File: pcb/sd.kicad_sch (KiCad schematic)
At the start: 1 part

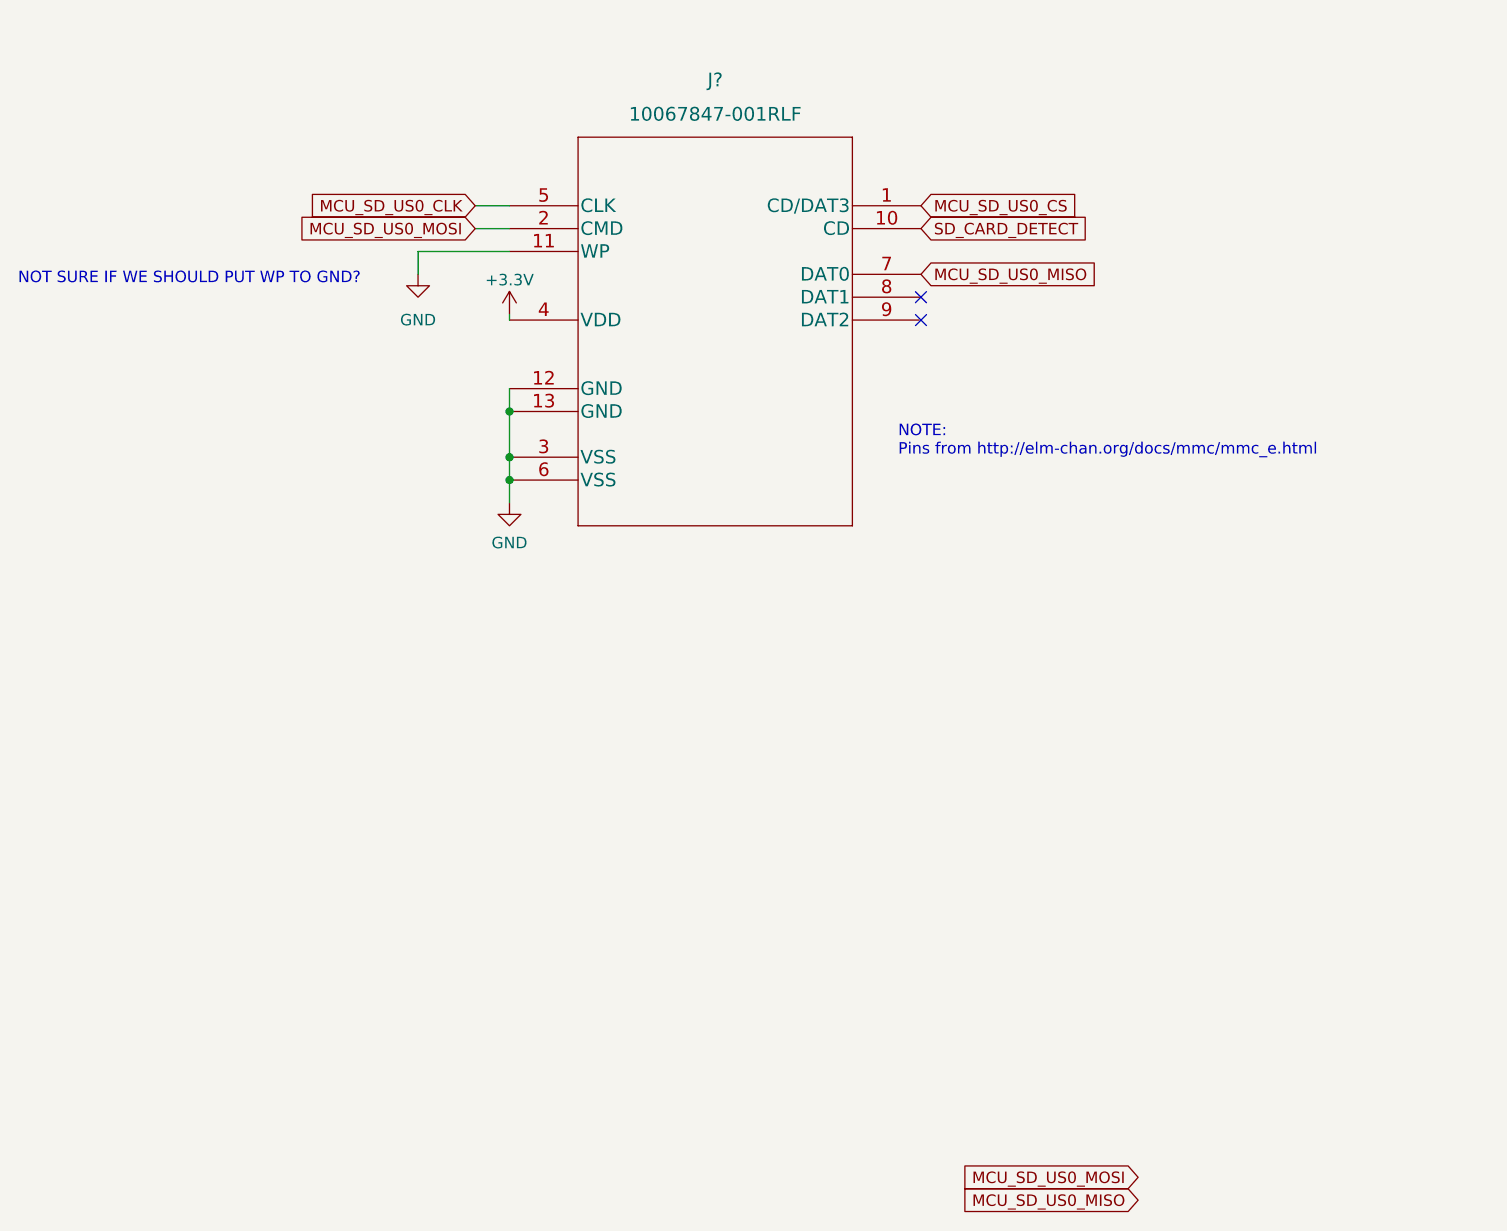
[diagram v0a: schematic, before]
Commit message: everything except crystal
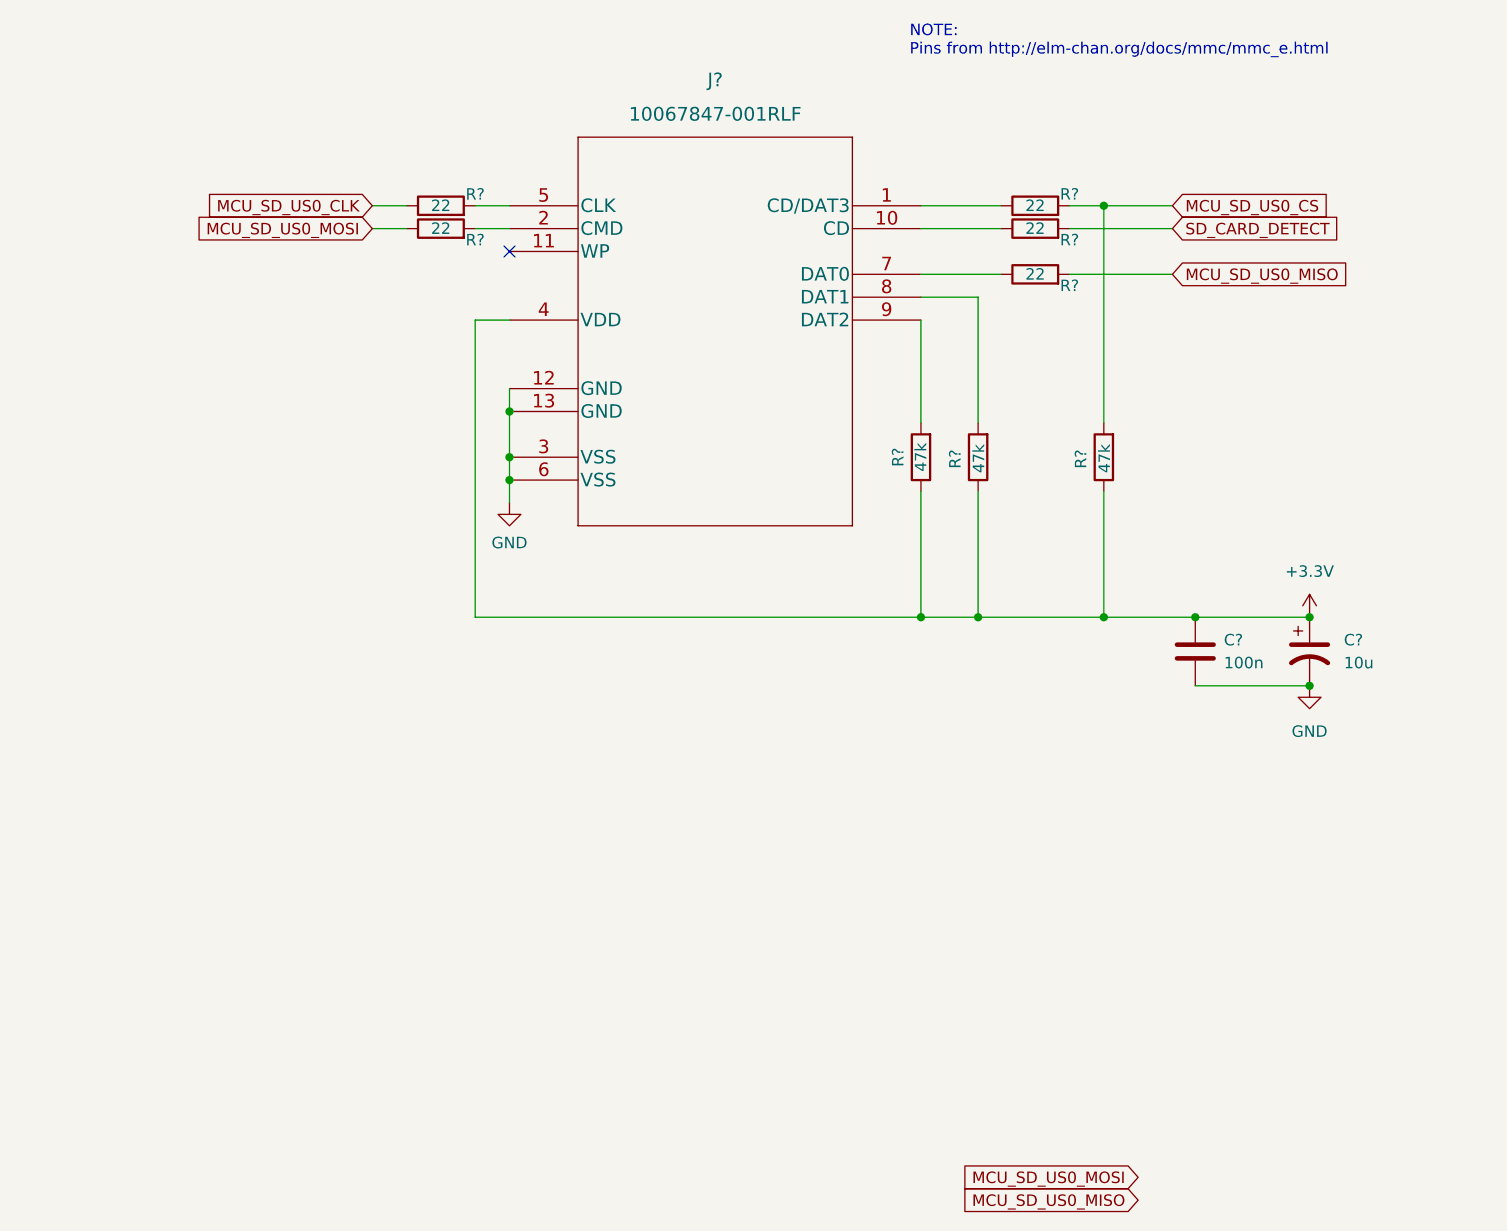
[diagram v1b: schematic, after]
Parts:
- added C?: 10u, symbol Device:C_Polarized_US
- added C?: 100n, symbol Device:C
- added R? (x5): 22, symbol Device:R
- added R? (x3): 47k, symbol Device:R
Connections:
- net +3.3V: now also C?.1, C?.1, R?.1, R?.1, R?.1
- net GND: now also C?.2, C?.2; no longer J?.11 (WP)
- net MCU_SD_US0_CLK: now also R?.1; no longer J?.5 (CLK)
- net MCU_SD_US0_CS: now also R?.2, R?.2; no longer J?.1 (CD/DAT3)
- net MCU_SD_US0_MISO: now also R?.2; no longer J?.7 (DAT0)
- net MCU_SD_US0_MOSI: now also R?.1; no longer J?.2 (CMD)
- net SD_CARD_DETECT: now also R?.2; no longer J?.10 (CD)
- net at J?.8 (DAT1): now also R?.2
- net at J?.9 (DAT2): now also R?.2
- new net: J?.1 (CD/DAT3), R?.1
- new net: J?.10 (CD), R?.1
- new net: J?.2 (CMD), R?.2
- new net: J?.5 (CLK), R?.2
- new net: J?.7 (DAT0), R?.1
- no-connect marks 2 -> 1
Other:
- note removed: "NOT SURE IF WE SHOULD PUT WP TO GND?"
